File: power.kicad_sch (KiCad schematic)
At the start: 36 parts, among them K1 G6K-2F-Y-TR, K2 G6K-2F-Y-TR, K3 G6K-2F-Y-TR, K4 G6K-2F-Y-TR, Q1 DMN2056U, Q2 DMN2056U, Q3 DMN2056U, Q4 DMN2056U, U2 TPS7A2401DBVR, U3 PI4IOE5V9536UEX

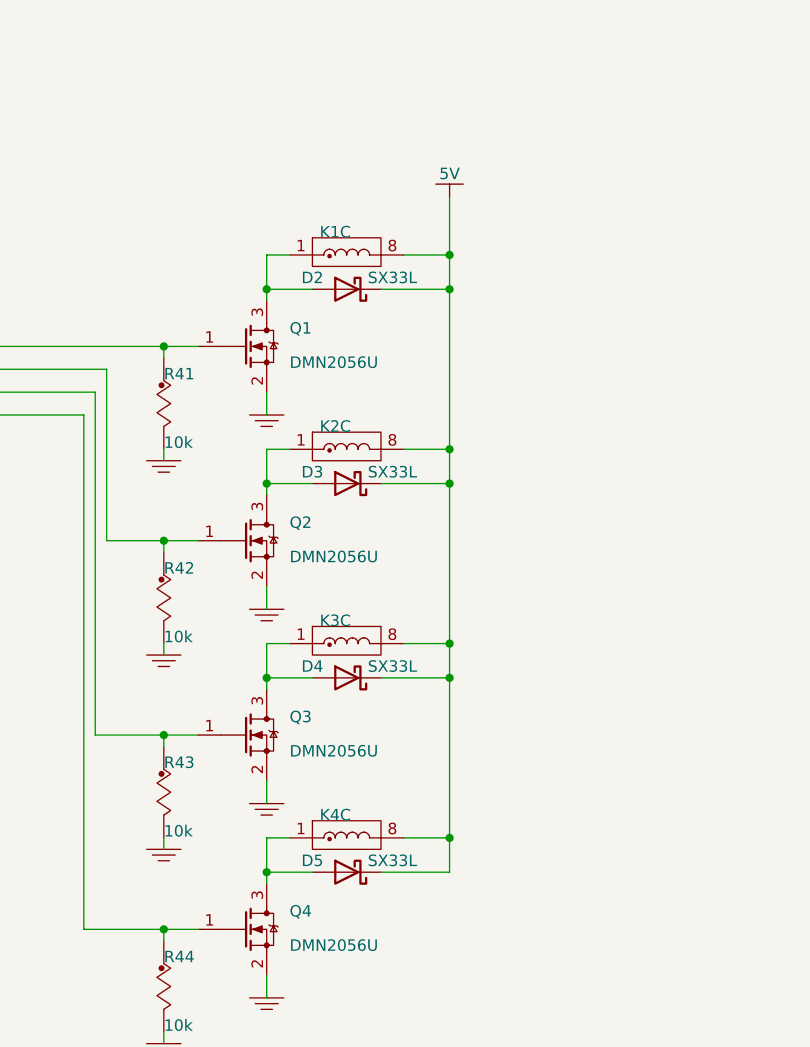
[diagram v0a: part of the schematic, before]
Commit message: Board is fully routed
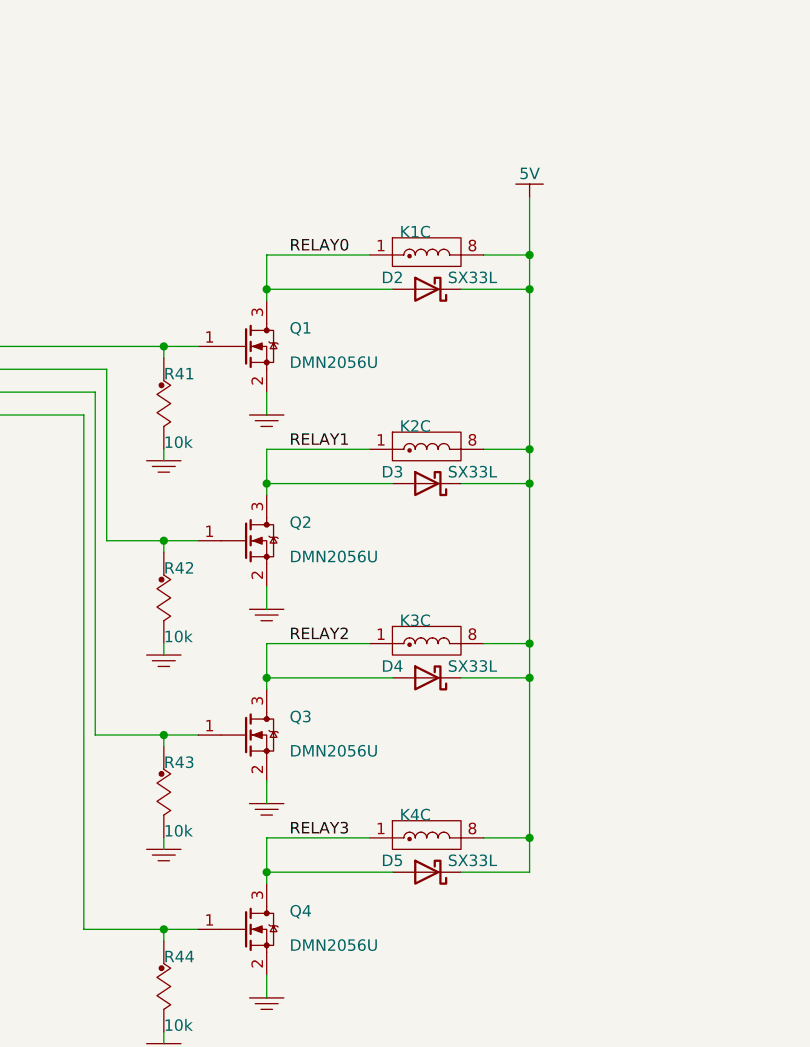
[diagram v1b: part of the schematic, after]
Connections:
- net RELAY3: now reaches D5.2 (A), K4.1 (COIL1), Q4.3 (D)
- net RELAY1: now reaches D3.2 (A), K2.1 (COIL1), Q2.3 (D)
- net RELAY0: now reaches D2.2 (A), K1.1 (COIL1), Q1.3 (D)
- net RELAY2: now reaches D4.2 (A), K3.1 (COIL1), Q3.3 (D)
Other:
- moved on the sheet: D2, D3, D4, D5, K1C, K2C, K3C, K4C
